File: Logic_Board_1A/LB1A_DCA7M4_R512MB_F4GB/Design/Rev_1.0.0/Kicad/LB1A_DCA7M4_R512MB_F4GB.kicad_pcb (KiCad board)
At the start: 6 copper layers, 50 x 50 mm, 143 parts, among them U1 STM32MP157CAC3, U2 AS4C256M16D3LC-12BCN, U3 S40FC004C1B2C00000, U4 STPMIC1BPQR, U5 DF40C-70DP-0.4V(51), U6 DF40C-70DP-0.4V(51), U7 DF40C-70DP-0.4V(51), X1 32.768kHz, X2 24MHz

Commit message: some more improvements
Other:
- net class DDR_DiffPairs: clearance 0.1016 -> 0.0762
- net class Default: clearance 0.1016 -> 0.0762
- net class Gnd_Lines: clearance 0.1016 -> 0.0762
- rule trace_clearance: 0.1016 -> 0.0762
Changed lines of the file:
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@@
   (page A4)
   (layers
-    (0 Top_Layer.Cu signal hide)
-    (1 Signal_Layer_1.Cu signal hide)
-    (2 Signal_Layer_2.Cu signal hide)
-    (3 Signal_Layer_3.Cu signal hide)
-    (4 Signal_Layer_4.Cu signal hide)
+    (0 Top_Layer.Cu signal)
+    (1 Signal_Layer_1.Cu signal)
+    (2 Signal_Layer_2.Cu signal)
+    (3 Signal_Layer_3.Cu signal)
+    (4 Signal_Layer_4.Cu signal)
     (31 Bottom_Layer.Cu signal)
     (32 B.Adhes user hide)
@@
     (user_trace_width 0.635)
     (user_trace_width 0.6604)
-    (trace_clearance 0.1016)
+    (trace_clearance 0.0762)
     (zone_clearance 0.1)
     (zone_45_only no)
@@
   (net 433 "Net-(U7-Pad58)")
   (net_class Default "This is the default net class."
-    (clearance 0.1016)
+    (clearance 0.0762)
     (trace_width 0.0889)
     (via_dia 0.40005)
@@
   )
   (net_class DDR_DiffPairs ""
-    (clearance 0.1016)
+    (clearance 0.0762)
     (trace_width 0.0889)
     (via_dia 0.40005)
@@
   )
   (net_class Gnd_Lines ""
-    (clearance 0.1016)
+    (clearance 0.0762)
     (trace_width 0.2032)
     (via_dia 0.40005)

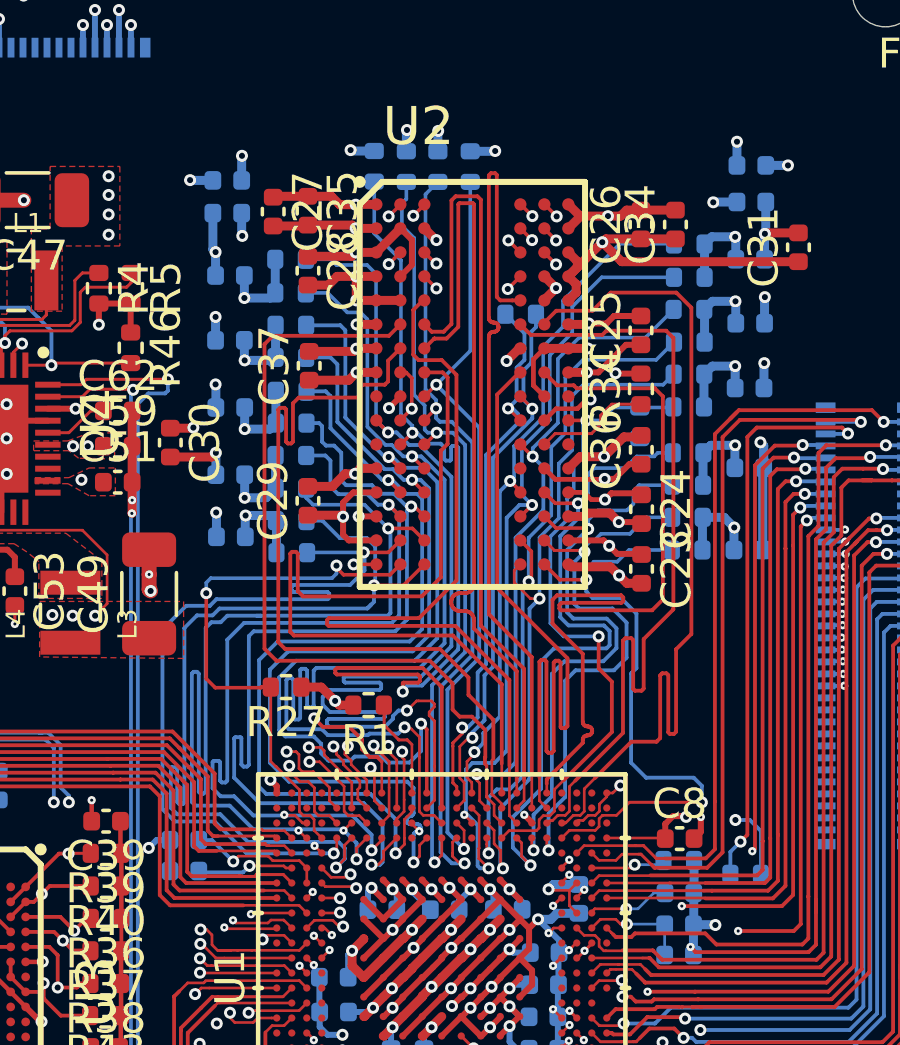
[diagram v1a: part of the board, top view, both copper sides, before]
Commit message: more imps
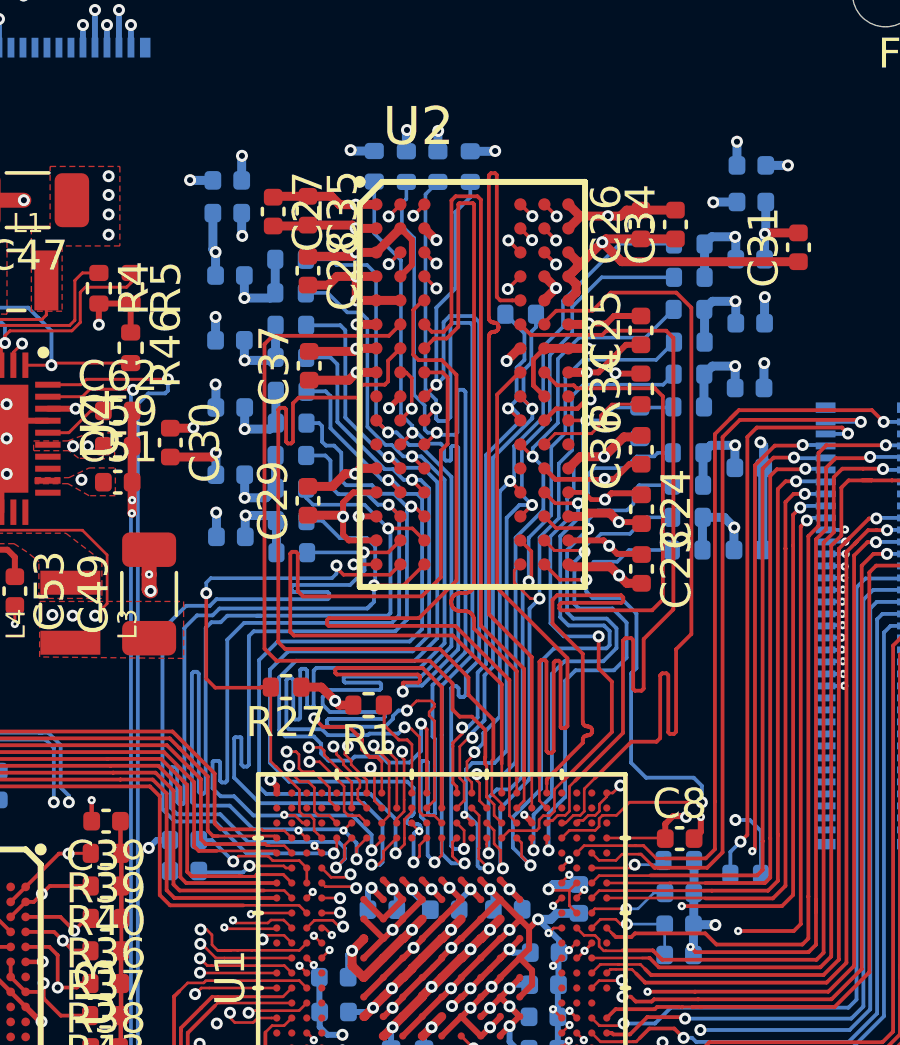
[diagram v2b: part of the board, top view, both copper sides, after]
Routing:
- net DDR_WEN: track 26.2 -> 33.3 mm
- net DDR_CASN: track 26.6 -> 33.4 mm
- net DDR_RASN: track 25.5 -> 31.6 mm
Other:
- net class DDR_DiffPairs: clearance 0.0762 -> 0.1016
- net class Default: clearance 0.0762 -> 0.1016
- net class Gnd_Lines: clearance 0.0762 -> 0.1016
- rule trace_clearance: 0.0762 -> 0.1016
